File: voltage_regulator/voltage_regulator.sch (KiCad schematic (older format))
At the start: 6 parts, among them Q1 BC548, U2 LM317AT

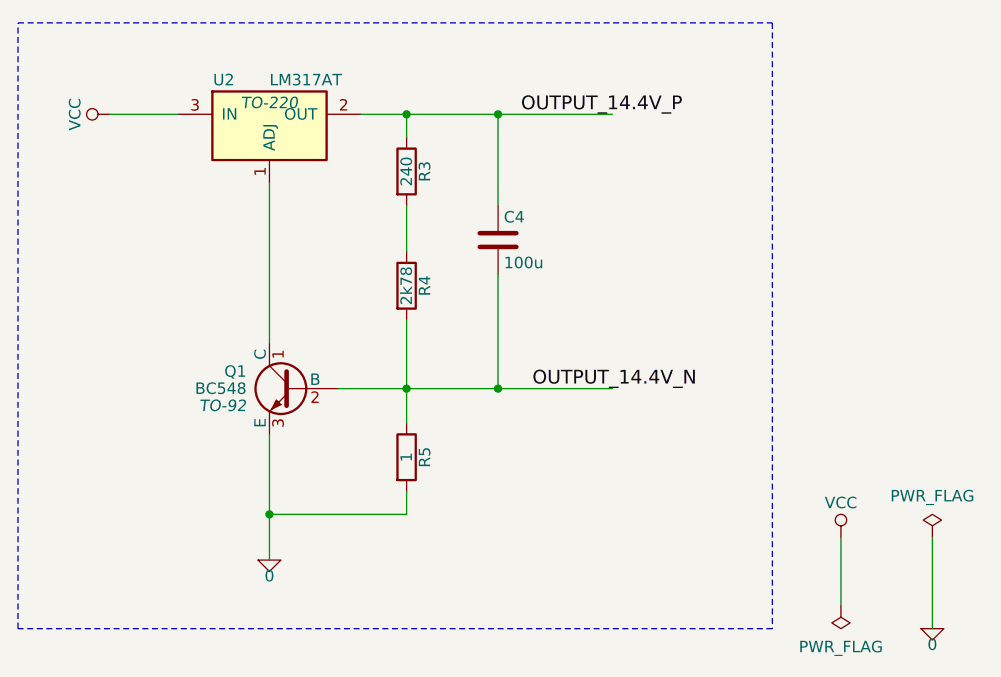
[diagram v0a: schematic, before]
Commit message: Design update
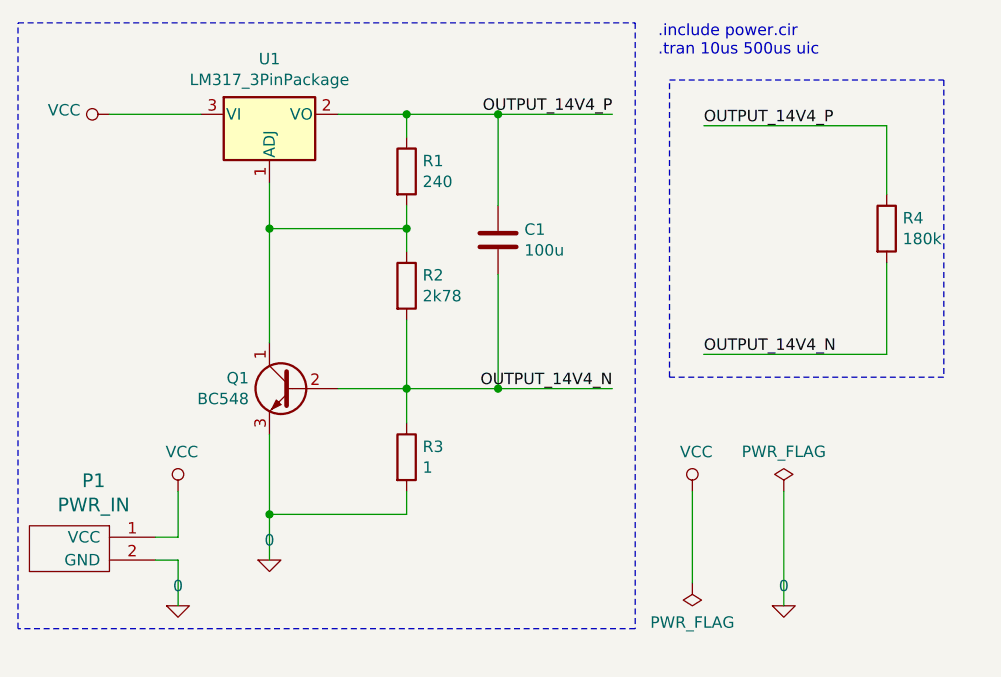
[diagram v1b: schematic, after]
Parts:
- removed C4: 100u, symbol voltage_regulator-rescue:C
- removed Q1: BC548, TO-92, symbol voltage_regulator-rescue:BC548
- removed R3: 240, symbol voltage_regulator-rescue:R
- removed R4: 2k78, symbol voltage_regulator-rescue:R
- removed R5: 1, symbol voltage_regulator-rescue:R
- removed U2: LM317AT, TO-220, symbol voltage_regulator-rescue:LM317AT
- added C1: 100u, symbol Device:C
- added P1: PWR_IN, symbol power_sources:PWR_IN
- added Q1: BC548, Package_TO_SOT_THT:TO-92_Inline, symbol Transistor_BJT:BC548
- added R1: 240, symbol Device:R
- added R2: 2k78, symbol Device:R
- added R3: 1, symbol Device:R
- added R4: 180k, symbol Device:R
- added U1: LM317_3PinPackage, symbol Regulator_Linear:LM317_3PinPackage
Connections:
- net labels added: OUTPUT_14V4_N, OUTPUT_14V4_P
- net labels removed: OUTPUT_14.4V_N, OUTPUT_14.4V_P
- wire segments 20 -> 31
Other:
- note added: ".include power.cir\n.tran 10us 500us uic"
